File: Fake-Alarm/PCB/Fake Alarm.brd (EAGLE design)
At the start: 30 x 33 mm, 15 parts, among them IC1 NE555DG4, X3 009176003

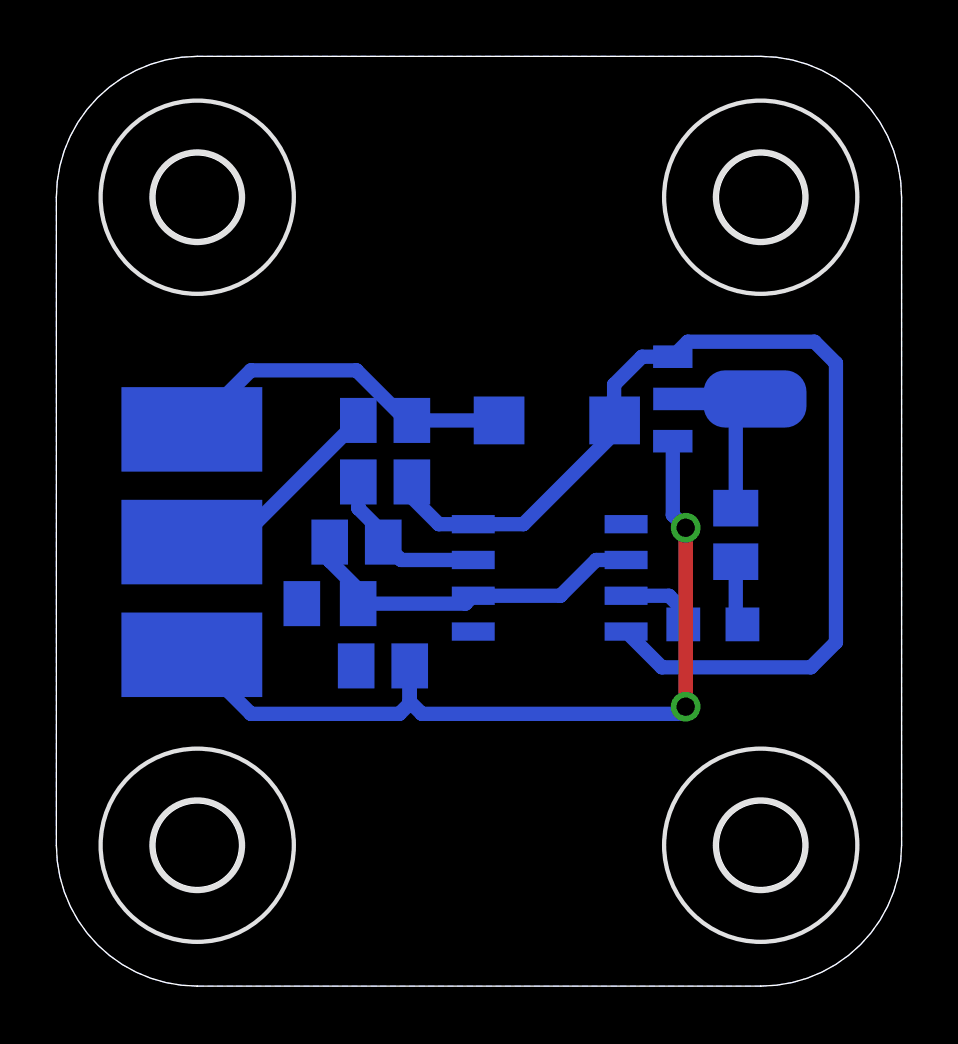
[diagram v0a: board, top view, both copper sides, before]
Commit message: Remove the OLD
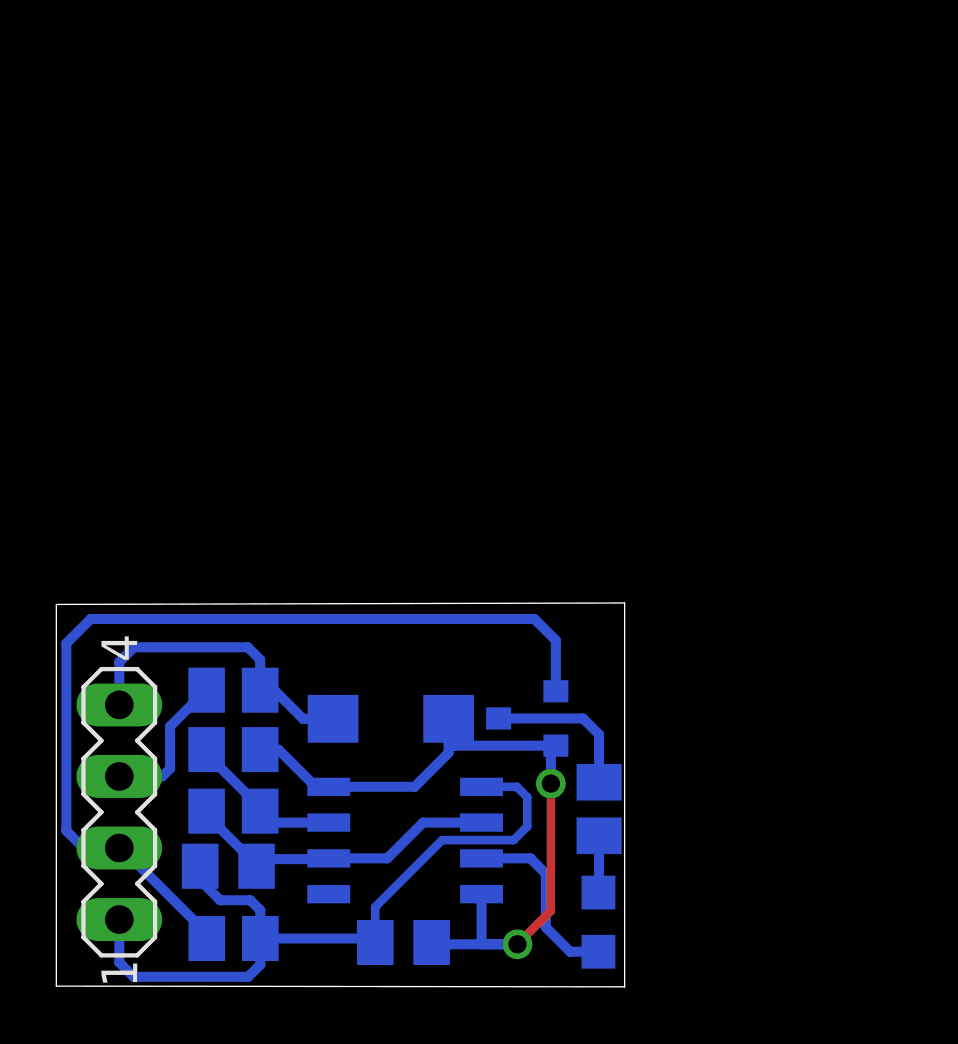
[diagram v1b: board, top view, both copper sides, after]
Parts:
- removed H1, H2, H3, H4: MOUNT-HOLE3.0, holes:3,0
- removed SS8550: (no value), zetex:SOT89
- removed X3: 009176003, con-avx:009176003
- added C2: 10uF, rcl:C0805K
- added SV1: (no value), con-lstb:MA04-1
- added T1: (no value), zetex:SOT-23
- R4: value (none) -> 10k
- moved 1N5819 12.1 mm to (11.9, 9.49)
- moved LED1 11.3 mm to (19.2, 2.27), turned to 180 degrees
- moved R4 11.0 mm to (6.29, 1.69), turned to 180 degrees
- moved R5 11.0 mm to (6.28, 10.5)
- moved R2 10.9 mm to (6.28, 8.39)
- moved R1 10.9 mm to (19.3, 6.29)
- moved IC1 10.6 mm to (12.4, 5.17)
- moved R3 10.5 mm to (6.28, 6.21)
- moved C1 10.00 mm to (6.11, 4.25)
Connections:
- net GND: now also C2.2, SV1.1
- net N$1: now also C2.1, T1.2; no longer SS8550.3
- net N$4: now also T1.1; no longer SS8550.2, SS8550.2@1
- net N$5: now also SV1.2, T1.3; no longer SS8550.1, X3.1
- net N$8: now also SV1.3; no longer X3.2
- net N$9: now also SV1.4; no longer X3.3
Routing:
- net GND: track 0.00 -> 26.7 mm
- net N$1: track 38.3 -> 27.3 mm, vias 0 -> 2
- net N$2: track 2.75 -> 6.64 mm
- net N$8: track 7.70 -> 5.53 mm
- net N$5: track 31.0 -> 33.2 mm, vias 2 -> 0
- net N$9: track 12.5 -> 11.0 mm
- net N$7: track 12.8 -> 11.3 mm
- net N$4: track 4.16 -> 5.50 mm
- removed copper zone on layer 16, net GND
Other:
- board size 30 x 33 mm -> 20.2 x 13.6 mm
